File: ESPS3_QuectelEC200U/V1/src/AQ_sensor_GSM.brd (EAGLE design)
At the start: 110 x 64 mm, 49 parts, among them IC2 MCP73831/OT, J1 F-1X03-SIP-100-32, SW1 PCM12SMTR, SW2 PCM12SMTR, U2 TEXAS_INSTRUMENTS_SN74HC125TE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, U3 TEXAS_INSTRUMENTS_LM1117IMP-3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, X1 53048-08, X2 SIMLOCK-C707_10M006_512_2, X4 50 Ohms

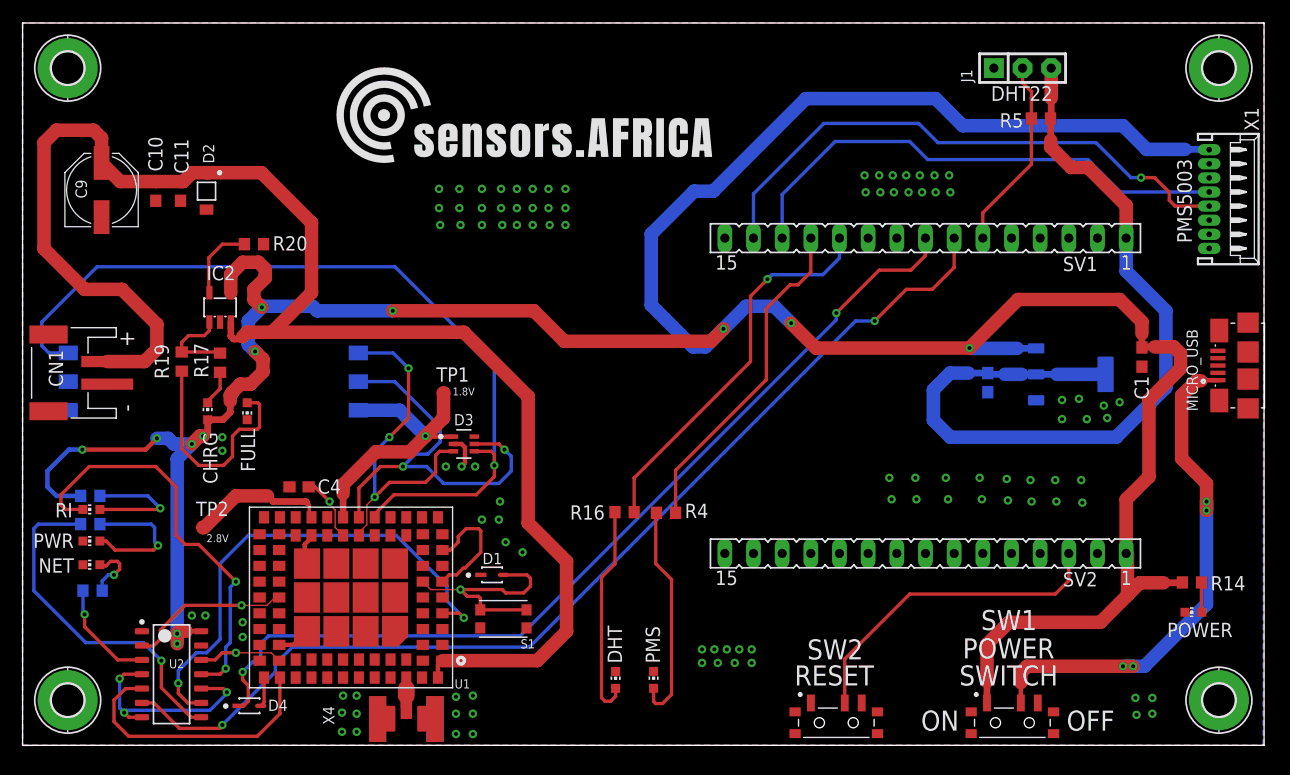
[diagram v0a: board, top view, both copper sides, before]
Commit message: V1 revised
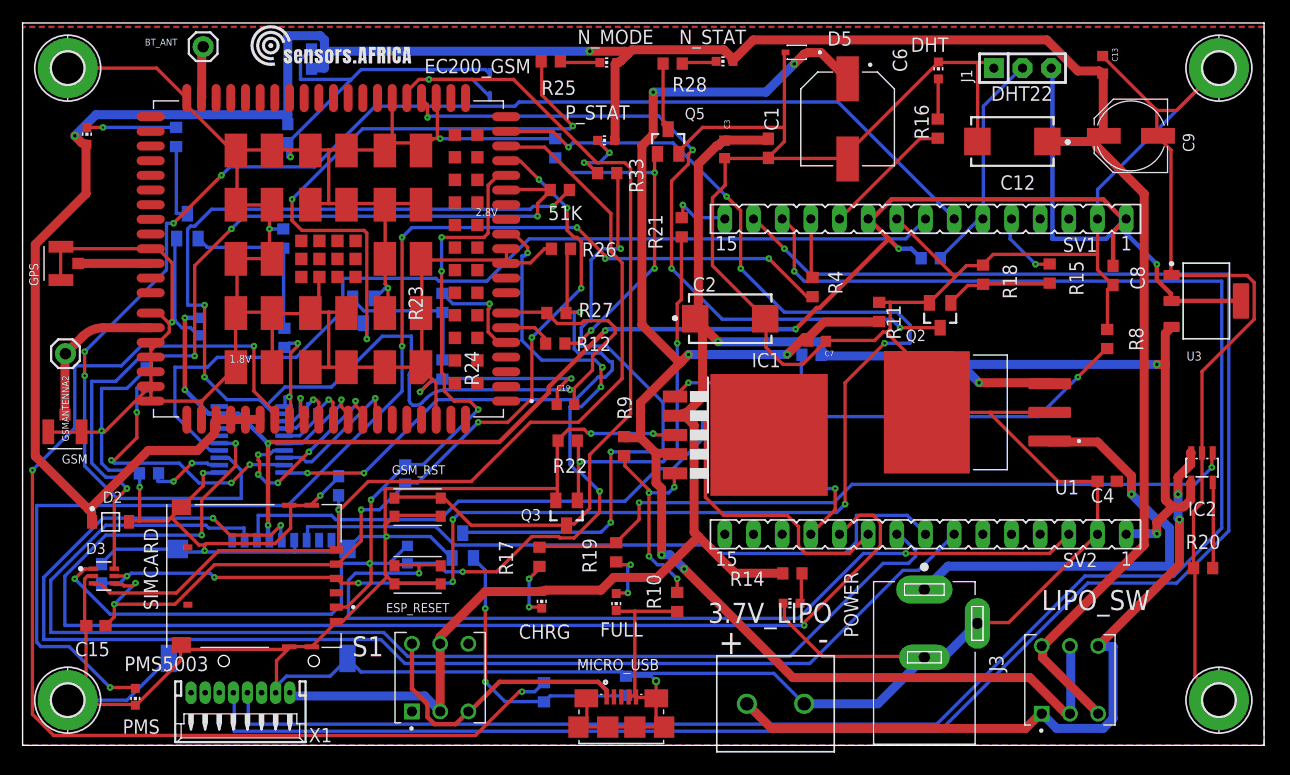
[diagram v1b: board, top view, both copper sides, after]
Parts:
- removed CN1: (no value), AQ_sensor_GSM:JST-PH-2-SMT-RA
- removed D4: ON_SEMI_1N4148WSON_SEMI_1N4148WS_0_0, AQ_sensor_GSM:ON_SEMI_1N4148WS_0
- removed NET: YELLOW, led:CHIP-LED0603
- removed PWR: RED, led:CHIP-LED0603
- removed R1, R6, R7: 470, rcl:R0603
- removed RI: ORANGE, led:CHIP-LED0603
- removed SW1, SW2: PCM12SMTR, AQ_sensor_GSM:SW_PCM12SMTR
- removed TP1, TP2: TPB1,27, testpad:B1,27
- removed U2: TEXAS_INSTRUMENTS_SN74HC125TEXAS_INSTRUMENTS_SN74HC125_0_0, AQ_sensor_GSM:TEXAS_INSTRUMENTS_SN74HC125_0
- removed X2: SIMLOCK-C707_10M006_512_2, AQ_sensor_GSM:C707_10M006_512_2
- removed X4: 50 Ohms, AQ_sensor_GSM:SMA_EDGELAUNCH_UFL
- added 10K, 51K, R12, R15, R21, R23, R3, R31, R34: 4.7K, rcl:R0603
- added 3.7V_LIPO: 2828XX-2282837-2, Connector:TERMBLK_508-2N
- added BT_ANT, GSMANTENNA2: (no value), SparkFun-Connectors:1X01
- added C12, C2: 470uf, T495X477K010ATE100:CAPMP7343X430N
- added C13, C18, C19, C20, C3, C7: 100nf, 06035C104K4T2A:CAPC1608X90N
- added C15, C16, C17: 33pF, rcl:C0603
- added C6: EEEFN1C471P, EEEFN1C471P:CAP_EEEFN1C471P
- added D5: ESD56151W04, 4.7V TVS Diode:DIO_1N4148WS_RR
- added EC200_GSM: EC200UCNAB-N05-SNNSA, EC200UCNAB-N05-SNNSA:XCVR_EC200UCNAB-N05-SNNSA
- added ESP_RESET, GSM_RST: KMR621NGLFS, AQ_sensor_GSM:SW_KMR621NGLFS
- added GPS, GSM: 1909763-1, 1909763-1:TE_1909763-1
- added IC1: MIC29302WU, MIC29302WU:TO263-5
- added J3: PJ-002BH, PJ-002BH:CUI_PJ-002BH
- added LIPO_SW: TL2285EE, TL2285EE:SW_TL2285EE
- added MICRO_SD1: TF-01A, TF-01A:TF-01A
- added M_RI, N_MODE, N_STAT, P_STAT: ORANGE, led:CHIP-LED0603
- added Q1, Q2, Q3, Q4, Q5, Q6, Q7: MMBT2222, MMBT2222_:SOT23-BEC
- added R10, R13, R18, R22, R24, R32, R35, R8: 47K, rcl:R0603
- added R11, R25, R28, R33, R36: 470R, rcl:R0603
- added R2, R29, R30: 51K, rcl:R0603
- added R26: 120K, rcl:R0603
- added R27: 10K, rcl:R0603
- added R9: 100k, rcl:R0603
- added SIMCARD: 78646-3001, 78646-3001:MOLEX_78646-3001
- added U5: TXS0108EPWR, TXS0108EPWR:SOP65P640X120-20N
- S1: value KMR621NGLFS -> TL2285EE; device AQ_sensor_GSM:SW_KMR621NGLFS -> TL2285EE:SW_TL2285EE
- U1: value (none) -> LM7805S/NOPB; device AQ_sensor_GSM:SIM800L -> LM7805S_NOPB:TO254P1524X483-4N
- moved X1 98.0 mm to (19.3, 3.41), turned to 180 degrees
- moved C9 91.3 mm to (98.2, 54.0), turned to 180 degrees
- moved R20 88.9 mm to (104.6, 15.7), turned to 180 degrees
- moved IC2 88.2 mm to (104.5, 24.6), turned to 180 degrees
- moved C4 71.6 mm to (96.1, 23.4)
- moved DHT 61.1 mm to (81.1, 59.8)
- moved MICRO_USB 60.5 mm to (53.0, 4.29), turned to 0 degrees
- moved U1 57.9 mm to (84.6, 29.5)
- moved PMS 45.9 mm to (9.99, 4.30), turned to 180 degrees
- moved R16 43.9 mm to (81.1, 54.6), turned to 270 degrees
- moved D1 43.4 mm to (41.4, 58.5), flipped to the bottom, turned to 270 degrees
- moved R19 42.0 mm to (52.6, 17.1)
- moved C1 37.9 mm to (66.1, 52.9)
- moved FULL 36.8 mm to (52.6, 12.7)
- moved POWER 35.6 mm to (68.1, 12.6)
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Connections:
- removed net 1.8V: D3.1, TP1.TP, U1.16, X2.C1
- removed net 2.8V: TP2.TP, U1.18
- removed net GSM_RX: D4.2, U1.31
- removed net GSM_RX_O: D4.1, SV1.8
- removed net GSM_TX: U1.32, U2.5
- removed net GSM_TX_5V: SV1.7, U2.6
- removed net N$10: NET.A, R6.2
- removed net N$11: PWR.A, R7.2
- removed net N$14: R1.2, RI.A
- removed net NETSTAT_5V: R6.1, U2.3
- removed net PWRSTAT_5V: R7.1, U2.8
- removed net RI: U1.68, U2.12
- removed net RI_5V: RI.C, U2.11
- removed net VBUS: U1.7
- removed net VIN: MICRO_USB.1, SW1.2
- new net BP: 3.7V_LIPO.2, IC2.3, LIPO_SW.1, LIPO_SW.6
- new net BT_ANT: BT_ANT.1, EC200_GSM.35
- new net CP: C6.1, C7.2, D5.C, IC1.4, LIPO_SW.2, LIPO_SW.5, R11.2, R9.2
- new net GNSS_ANT: EC200_GSM.47, GPS.1
- new net JACKP: J3.1, U1.1
- new net MAIN_CTS: EC200_GSM.64, U5.4
- new net MAIN_DCD: EC200_GSM.63, U5.3
- new net MAIN_DTR: EC200_GSM.66, U5.6
- new net MAIN_RI: EC200_GSM.62, R34.1, U5.1
- new net MAIN_RTS: EC200_GSM.65, U5.5
- new net MAIN_RXD: EC200_GSM.68, U5.8
- new net MAIN_TXD: EC200_GSM.67, U5.7
- new net MCU_CTS: U5.17
- new net MCU_DCD: U5.18
- new net MCU_DTR: SV2.11, U5.15
- new net MCU_RI: U5.20
- new net MCU_RTS: U5.16
- new net MCU_RXD: SV1.8, U5.14
- new net MCU_TXD: SV1.7, U5.13
- new net N$1: Q2.B, R15.2, R18.2
- new net N$15: EC200_GSM.127
- new net N$16: EC200_GSM.135
- new net N$2: Q3.B, R21.2, R22.2
- new net N$22: Q5.B, R12.2, R13.2
- new net N$23: EC200_GSM.2
- new net N$26: Q4.B, R23.2, R24.2
- new net N$28: Q6.B, R31.2, R32.2
- new net N$29: Q4.C, R25.1
- new net N$30: N_MODE.C, R25.2
- new net N$31: R26.1, R27.2, U5.10
- new net N$32: Q6.C, R33.1
- new net N$33: Q5.C, R28.1
- new net N$34: N_STAT.C, R28.2
- new net N$35: IC1.1, Q1.C, R2.1
- new net N$36: Q1.B, R3.2
- new net N$37: Q1.E, R8.2
- new net N$38: IC1.5, R10.2, R9.1
- new net N$39: P_STAT.C, R33.2
- new net N$40: R30.1, U5.9
- new net N$41: R29.1, U5.12
- new net N$42: Q7.B, R34.2, R35.2
- new net N$43: Q7.C, R36.1
- new net N$44: M_RI.C, R36.2
- new net N$5: EC200_GSM.128
- new net N$7: EC200_GSM.139
- new net N$8: EC200_GSM.136
- new net NET_MODE: EC200_GSM.5, R23.1
- new net PWRKEY_0: R21.1, SV1.15
- new net SDIO1_VDD: EC200_GSM.34
- new net TF-CLK: MICRO_SD1.5, SV2.7
- new net TF-CS: MICRO_SD1.2, SV2.9
- new net TF-MISO: MICRO_SD1.7, SV2.8
- new net TF-MOSI: MICRO_SD1.3, SV2.10
- new net USBP: MICRO_USB.1, S1.3, S1.4
- new net USB_VBUS: EC200_GSM.71
- new net USIM_DET: 51K.1, D3.6, EC200_GSM.13
- new net USIM_GND: C18.1, EC200_GSM.10
- new net USIM_VDD: 10K.2, C18.2, D3.1, EC200_GSM.14, SIMCARD.C1
- new net VBAT_EN: R3.1, SV2.12
- new net VDD_EXT: 51K.2, C19.2, EC200_GSM.7, R27.1, U5.2
- new net VPP: SIMCARD.C6
- net +3V3: now also C20.2, MICRO_SD1.4, SV1.10, U5.19
- net +5V: now also C2.1, C3.2, IC1.2, R2.2, S1.2, S1.5, U1.3; no longer R1.1, SW1.1, U2.14
- net ESP_RST: now also ESP_RESET.2_1, ESP_RESET.2_2; no longer SW2.2
- net GND: now also 3.7V_LIPO.1, C12.2, C13.1, C15.2, C16.2, C17.2, C19.1, C2.2, C20.1, C3.1, C6.2, C7.1, D5.A, EC200_GSM.100, EC200_GSM.101, EC200_GSM.102, EC200_GSM.103, EC200_GSM.104, EC200_GSM.105, EC200_GSM.106, EC200_GSM.107, EC200_GSM.108, EC200_GSM.109, EC200_GSM.110, EC200_GSM.111, EC200_GSM.112, EC200_GSM.19, EC200_GSM.22, EC200_GSM.36, EC200_GSM.46, EC200_GSM.48, EC200_GSM.50, EC200_GSM.51, EC200_GSM.52, EC200_GSM.53, EC200_GSM.54, EC200_GSM.56, EC200_GSM.72, EC200_GSM.76, EC200_GSM.8, EC200_GSM.85, EC200_GSM.86, EC200_GSM.87, EC200_GSM.88, EC200_GSM.89, EC200_GSM.9, EC200_GSM.90, EC200_GSM.91, EC200_GSM.92, EC200_GSM.93, EC200_GSM.94, EC200_GSM.95, EC200_GSM.96, EC200_GSM.97, EC200_GSM.98, EC200_GSM.99, ESP_RESET.1_1, ESP_RESET.1_2, GPS.2, GPS.3, GSM.2, GSM.3, GSM_RST.1_1, GSM_RST.1_2, IC1.3, J3.2, J3.3, MICRO_SD1.6, MICRO_SD1.MP1, MICRO_SD1.MP2, MICRO_SD1.MP3, MICRO_SD1.MP4, Q2.E, Q3.E, Q4.E, Q5.E, Q6.E, Q7.E, R10.1, R11.1, R13.1, R18.1, R22.1, R24.1, R26.2, R29.2, R30.2, R32.1, R35.1, R8.1, SIMCARD.C5, SIMCARD.G1, SIMCARD.G2, SIMCARD.G3, SIMCARD.G4, SIMCARD.G5, SIMCARD.G6, SV1.9, U1.4, U5.11; no longer CN1.2, NET.C, PWR.C, S1.1_1, S1.1_2, SW1.S1, SW1.S2, SW1.S3, SW1.S4, SW2.1, SW2.S1, SW2.S2, SW2.S3, SW2.S4, U1.35, U1.37, U1.38, U1.39, U1.41, U1.43, U1.44, U1.45, U1.58, U1.6, U1.67, U1.71, U1.72, U1.73, U1.76, U1.77, U1.78, U1.79, U1.8, U1.80, U1.81, U1.82, U1.83, U1.84, U1.85, U1.86, U1.87, U1.88, U2.1, U2.10, U2.13, U2.4, U2.7, X2.C5, X4.GND@1, X4.GND@2, X4.GND@3, X4.GND@4
- net GSM_ANT: now also EC200_GSM.49, GSM.1, GSMANTENNA2.1; no longer U1.40, X4.P
- net GSM_RST: now also EC200_GSM.20, Q2.C; no longer U1.49
- net GSM_RST_O: now also R15.1
- net NETSTAT: now also EC200_GSM.6, R12.1; no longer U1.64, U2.2
- net PWRKEY: now also EC200_GSM.21, GSM_RST.2_1, GSM_RST.2_2, Q3.C; no longer S1.2_1, S1.2_2, U1.48
- net PWRSTAT: now also EC200_GSM.61, R31.1; no longer U1.4, U2.9
- net SIMCLK: now also C16.1, EC200_GSM.16, SIMCARD.C3; no longer U1.55, X2.C3
- net SIMDATA: now also 10K.1, C15.1, EC200_GSM.15, SIMCARD.C7; no longer U1.14, X2.C7
- net SIMRST: now also C17.1, EC200_GSM.17, SIMCARD.C2; no longer U1.15, X2.C2
- net VRTC: no longer U1.56
- net V_LIPO: now also C12.1, C13.2, EC200_GSM.57, EC200_GSM.58, EC200_GSM.59, EC200_GSM.60, LIPO_SW.3, LIPO_SW.4, M_RI.A, N_MODE.A, N_STAT.A, P_STAT.A; no longer CN1.1, IC2.3, U1.1, U1.42
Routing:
- net GND: track 39.1 -> 872.6 mm, vias 103 -> 16
- net CP: track 0.00 -> 135.6 mm, vias 0 -> 6
- net MCU_TXD: track 0.00 -> 123.0 mm, vias 0 -> 4
- net TF-CLK: track 0.00 -> 117.3 mm, vias 0 -> 2
- net PMS_RX: track 45.5 -> 161.5 mm, vias 0 -> 1
- net PMS_TX: track 50.3 -> 165.8 mm
- net VDD_EXT: track 0.00 -> 113.4 mm, vias 0 -> 4
- net MCU_DTR: track 0.00 -> 110.8 mm, vias 0 -> 3
- net TF-CS: track 0.00 -> 109.0 mm
- net +5V: track 283.1 -> 177.2 mm, vias 12 -> 4
- net V_LIPO: track 136.5 -> 241.5 mm, vias 0 -> 2
- net SIMRST: track 37.4 -> 139.6 mm, vias 2 -> 10
- net GSM_TX_5V: track 92.9 -> 0.00 mm, vias 2 -> 0
- net N$4: track 19.9 -> 112.1 mm, vias 0 -> 6
- net USIM_VDD: track 0.00 -> 89.6 mm, vias 0 -> 6
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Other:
- board text added: "+"
- board text added: "-"
- board text added: "/Users/augustinemwendwa/Downloads/Logo-Files-01 (2) (1) (1).bmp"
- board text added: "/Users/augustinemwendwa/Downloads/Logo-Files-01 (2) (1).bmp"
- board text removed: "/Users/kirah/Downloads/Logo-Files-01.bmp"
- board text removed: "OFF"
- board text removed: "ON"
- board text removed: "POWER"
- board text removed: "RESET"
- board text removed: "SWITCH"
